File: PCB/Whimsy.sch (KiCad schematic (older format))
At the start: 3 parts, among them J1 OLED, J2 LED Breakout, U1 Elite-C

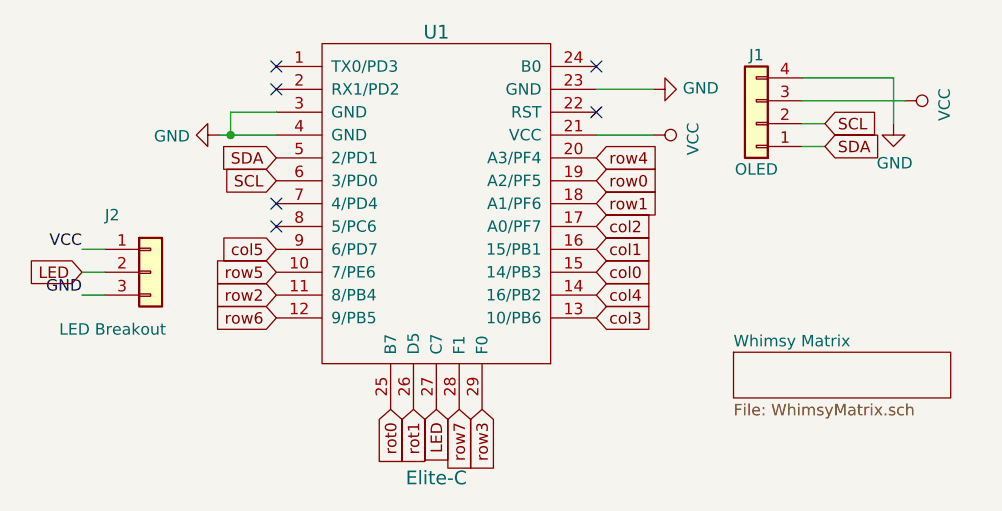
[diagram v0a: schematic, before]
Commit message: updated PCB design
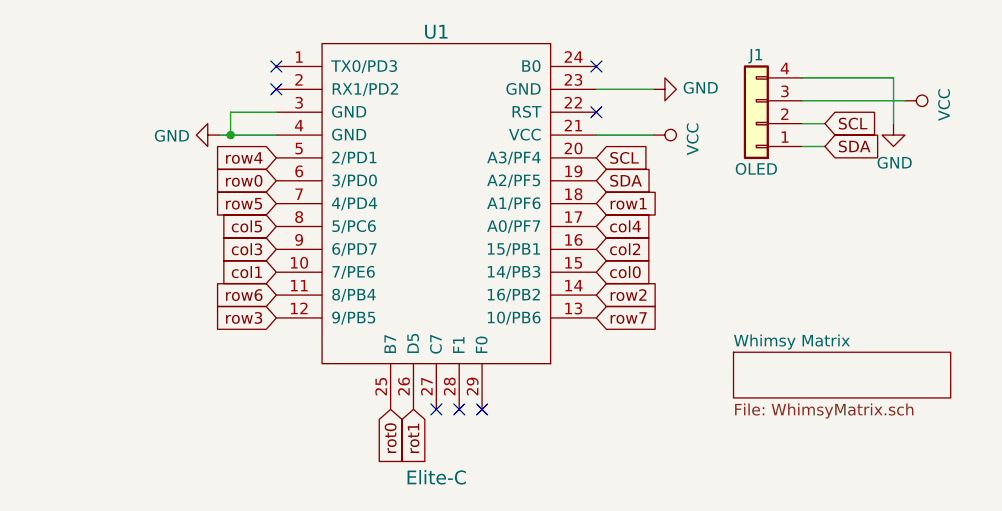
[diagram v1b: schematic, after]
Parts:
- removed J2: LED Breakout, SofleKeyboard-footprint:LED, symbol Connector_Generic:Conn_01x03
- J1: footprint SofleKeyboard-footprint:OLED_4Pin -> CustomPrints:OLED_4Pin
- U1: footprint Keebio-Parts:Elite-C-NoSilk -> CustomPrints:Elite-C-NoSilk
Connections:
- net SCL: now also U1.20 (A3/PF4); no longer U1.6 (3/PD0)
- net SDA: now also U1.19 (A2/PF5); no longer U1.5 (2/PD1)
- net col1: now also U1.10 (7/PE6); no longer U1.16 (15/PB1)
- net col2: now also U1.16 (15/PB1); no longer U1.17 (A0/PF7)
- net col3: now also U1.9 (6/PD7); no longer U1.13 (10/PB6)
- net col4: now also U1.17 (A0/PF7); no longer U1.14 (16/PB2)
- net col5: now also U1.8 (5/PC6); no longer U1.9 (6/PD7)
- net row0: now also U1.6 (3/PD0); no longer U1.19 (A2/PF5)
- net row2: now also U1.14 (16/PB2); no longer U1.11 (8/PB4)
- net row3: now also U1.12 (9/PB5); no longer U1.29 (F0)
- net row4: now also U1.5 (2/PD1); no longer U1.20 (A3/PF4)
- net row5: now also U1.7 (4/PD4); no longer U1.10 (7/PE6)
- net row6: now also U1.11 (8/PB4); no longer U1.12 (9/PB5)
- net row7: now also U1.13 (10/PB6); no longer U1.28 (F1)
- net LED: no longer names the net of U1.27 (C7)
- no-connect marks 6 -> 7
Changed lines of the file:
@@
 F 0 "J1" H 5800 3300 50  0000 C CNN
 F 1 "OLED" H 5800 3800 50  0000 C CNN
-F 2 "SofleKeyboard-footprint:OLED_4Pin" H 5800 3600 50  0001 C CNN
+F 2 "CustomPrints:OLED_4Pin" H 5800 3600 50  0001 C CNN
 F 3 "~" H 5800 3600 50  0001 C CNN
 	1    5800 3600
 	-1   0    0    1
 $EndComp
-Text GLabel 3700 3750 0    50   Input ~ 0
+Text GLabel 5100 3850 2    50   Input ~ 0
 SDA
-Text GLabel 3700 3850 0    50   Input ~ 0
+Text GLabel 5100 3750 2    50   Input ~ 0
 SCL
 Text GLabel 5100 4250 2    50   Input ~ 0
 col0
+Text GLabel 3700 4250 0    50   Input ~ 0
+col1
 Text GLabel 5100 4150 2    50   Input ~ 0
-col1
-Text GLabel 5100 4050 2    50   Input ~ 0
 col2
-Text GLabel 5100 4450 2    50   Input ~ 0
+Text GLabel 3700 4150 0    50   Input ~ 0
 col3
-Text GLabel 5100 3850 2    50   Input ~ 0
+Text GLabel 3700 3850 0    50   Input ~ 0
 row0
 Text GLabel 5100 3950 2    50   Input ~ 0
 row1
+Text GLabel 5100 4350 2    50   Input ~ 0
+row2
+Text GLabel 3700 4450 0    50   Input ~ 0
+row3
+Text GLabel 3700 3750 0    50   Input ~ 0
+row4
+Text GLabel 3700 3950 0    50   Input ~ 0
+row5
 Text GLabel 3700 4350 0    50   Input ~ 0
-row2
-Text GLabel 4600 4850 3    50   Input ~ 0
-row3
-Text GLabel 5100 3750 2    50   Input ~ 0
-row4
-Text GLabel 3700 4250 0    50   Input ~ 0
-row5
-Text GLabel 3700 4450 0    50   Input ~ 0
 row6
-Text GLabel 4500 4850 3    50   Input ~ 0
+Text GLabel 5100 4450 2    50   Input ~ 0
 row7
-Text GLabel 5100 4350 2    50   Input ~ 0
+Text GLabel 5100 4050 2    50   Input ~ 0
 col4
-Text GLabel 3700 4150 0    50   Input ~ 0
+Text GLabel 3700 4050 0    50   Input ~ 0
 col5
-$Comp
-L Connector_Generic:Conn_01x03 J2
-U 1 1 5E7C12A5
-P 3150 4250
-F 0 "J2" H 2950 4500 50  0000 L CNN
-F 1 "LED Breakout" H 2750 4000 50  0000 L CNN
-F 2 "SofleKeyboard-footprint:LED" H 3150 4250 50  0001 C CNN
-F 3 "~" H 3150 4250 50  0001 C CNN
-	1    3150 4250
-	1    0    0    -1
-$EndComp
-Text Label 2850 4150 2    50   ~ 0
-VCC
-Text Label 2850 4350 2    50   ~ 0
-GND
-Wire Wire Line
-	2850 4150 2950 4150
-Wire Wire Line
-	2950 4250 2850 4250
-Wire Wire Line
-	2950 4350 2850 4350
 Text GLabel 4200 4850 3    50   Input ~ 0
 rot0
@@
 F 0 "U1" H 4400 4600 60  0000 C CNN
 F 1 "Elite-C" H 4400 2650 60  0000 C CNN
-F 2 "Keebio-Parts:Elite-C-NoSilk" V 5450 1400 60  0001 C CNN
+F 2 "CustomPrints:Elite-C-NoSilk" V 5450 1400 60  0001 C CNN
 F 3 "" V 5450 1400 60  0001 C CNN
 	1    4400 3900
@@
 Wire Wire Line
 	5100 3650 5350 3650
-NoConn ~ 3700 4050
-NoConn ~ 3700 3950
+NoConn ~ 4600 4850
+NoConn ~ 4500 4850
 NoConn ~ 5100 3350
 NoConn ~ 3700 3450
 NoConn ~ 3700 3350
 NoConn ~ 5100 3550
-Text GLabel 2850 4250 0    50   Input ~ 0
-LED
-Text GLabel 4400 4850 3    50   Input ~ 0
-LED
 $Comp
 L power:GND #PWR0101
@@
 	1    0    0    -1
 $EndComp
+NoConn ~ 4400 4850
 $EndSCHEMATC
